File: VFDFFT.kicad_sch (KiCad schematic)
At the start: 278 parts, among them J1 USB_C_Receptacle_USB2.0, J10 Conn_01x02_Pin, J11 Conn_01x02_Male, J12 Conn_01x02_Male, J13 Conn_01x02_Male, J14 AudioJack3_Ground, J15 USB_C_Receptacle_USB2.0, J2 BATT, J3 FILAMENT+, J4 VFD_SIG, J5 USB_A, J6 Conn_01x03_Socket, J7 Conn_01x03_Socket, J8 Conn_01x02_Pin, J9 Conn_01x02_Pin, Q1 IRL7486MTRPBF, Q10 AO3400A, Q11 AO3400A, Q12 FS5N10S, Q2 ASDM30DN40E, Q3 ASDM30DN40E, Q4 HSCB2903, Q5 HSCB2903, Q6 AP6800, Q7 FS5N10S, Q8 FS5N10S, Q9 AO3400A, U1 IP2368, U10 TPS61170, U11 TPS61170, U12 W25Q128JVS, U13 TPS62170DSG, U14 LM358, U15 LM324, U16 LM3478, U17 LM2738, U18 ES9023, U19 CH340E, U2 78L05_SOT23, U3 TPS40305, U4 LM3478, U5 LM3478, U6 STM32F446VETx, U7 AP6181, U8 HDC1080, U9 OPT3001DNPR, X1 SX1M32.768KM10F30TNN, Y1 WTL3M45404LZ, Y2 24M

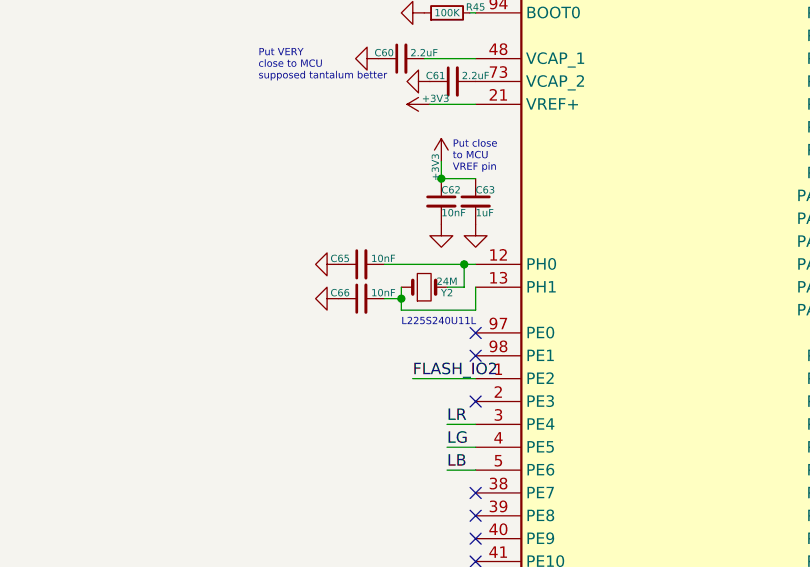
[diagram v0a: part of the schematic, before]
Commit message: file sync
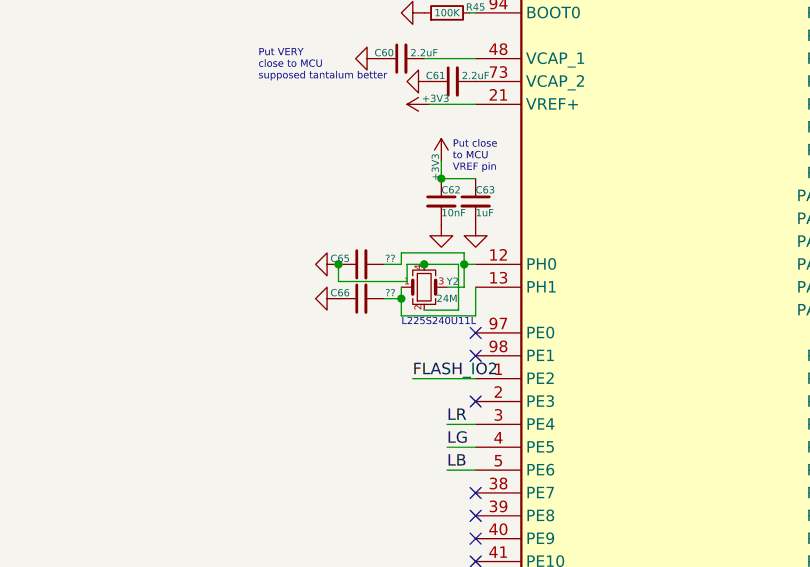
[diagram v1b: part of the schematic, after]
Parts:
- removed Y2: 24M, Resistor_SMD:R_0805_2012Metric, symbol Device:Crystal_Small
- added Y2: 24M, Crystal:Crystal_SMD_3225-4Pin_3.2x2.5mm, symbol Device:Crystal_GND24_Small
- C65, C66: value 10nF -> ??
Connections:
- net GND: now also Y2.2, Y2.4
- net at C66.2, U6.13 (PH1): now also Y2.1
- net at C65.2, U6.12 (PH0): now also Y2.3
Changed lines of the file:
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@@
   (junction (at 58.42 175.26) (diameter 0) (color 0 0 0 0)
   )
+  (junction (at 293.37 78.74) (diameter 0) (color 0 0 0 0)
+  )
   (junction (at 104.775 25.4) (diameter 0) (color 0 0 0 0)
   )
@@
   (junction (at 168.275 269.875) (diameter 0) (color 0 0 0 0)
   )
+  (junction (at 283.845 78.74) (diameter 0) (color 0 0 0 0)
+  )
   (junction (at 40.005 97.79) (diameter 0) (color 0 0 0 0)
   )
@@
     (stroke (width 0) (type default))
   )
+  (wire (pts (xy 291.465 78.74) (xy 291.465 80.645))
+    (stroke (width 0) (type default))
+  )
   (wire (pts (xy 199.39 241.935) (xy 202.565 241.935))
     (stroke (width 0) (type default))
@@
     (stroke (width 0) (type default))
   )
+  (wire (pts (xy 290.83 78.74) (xy 288.925 78.74))
+    (stroke (width 0) (type default))
+  )
   (wire (pts (xy 169.545 239.395) (xy 190.5 239.395))
     (stroke (width 0) (type default))
@@
     (stroke (width 0) (type default))
   )
-  (wire (pts (xy 299.085 81.28) (xy 299.085 83.82))
+  (wire (pts (xy 299.085 81.28) (xy 299.085 84.455))
     (stroke (width 0) (type default))
   )
@@
     (stroke (width 0) (type default))
   )
+  (wire (pts (xy 297.18 83.82) (xy 297.18 78.74))
+    (stroke (width 0) (type default))
+  )
   (wire (pts (xy 64.135 99.695) (xy 64.135 100.33))
     (stroke (width 0) (type default))
@@
     (stroke (width 0) (type default))
   )
+  (wire (pts (xy 293.37 78.74) (xy 291.465 78.74))
+    (stroke (width 0) (type default))
+  )
   (wire (pts (xy 75.565 119.38) (xy 75.565 121.92))
     (stroke (width 0) (type default))
@@
     (stroke (width 0) (type default))
   )
+  (wire (pts (xy 293.37 83.82) (xy 297.18 83.82))
+    (stroke (width 0) (type default))
+  )
   (wire (pts (xy 210.82 168.91) (xy 210.82 169.545))
     (stroke (width 0) (type default))
   )
+  (wire (pts (xy 297.815 77.47) (xy 297.815 78.74))
+    (stroke (width 0) (type default))
+  )
   (wire (pts (xy 175.26 275.59) (xy 187.96 275.59))
     (stroke (width 0) (type default))
@@
     (stroke (width 0) (type default))
   )
-  (wire (pts (xy 290.83 83.82) (xy 290.83 82.55))
+  (wire (pts (xy 290.83 84.455) (xy 290.83 82.55))
     (stroke (width 0) (type default))
   )
@@
     (stroke (width 0) (type default))
   )
+  (wire (pts (xy 283.845 80.645) (xy 283.845 78.74))
+    (stroke (width 0) (type default))
+  )
   (wire (pts (xy 57.15 111.76) (xy 57.15 112.395))
     (stroke (width 0) (type default))
@@
     (stroke (width 0) (type default))
   )
-  (wire (pts (xy 288.925 78.74) (xy 297.815 78.74))
+  (wire (pts (xy 290.83 77.47) (xy 297.815 77.47))
     (stroke (width 0) (type default))
   )
@@
     (stroke (width 0) (type default))
   )
+  (wire (pts (xy 290.83 77.47) (xy 290.83 78.74))
+    (stroke (width 0) (type default))
+  )
   (wire (pts (xy 295.275 116.84) (xy 299.085 116.84))
     (stroke (width 0) (type default))
@@
     (stroke (width 0) (type default))
   )
+  (wire (pts (xy 297.18 78.74) (xy 293.37 78.74))
+    (stroke (width 0) (type default))
+  )
   (wire (pts (xy 73.66 252.73) (xy 73.66 264.16))
     (stroke (width 0) (type default))
@@
     (stroke (width 0) (type default))
   )
-  (wire (pts (xy 299.085 83.82) (xy 290.83 83.82))
+  (wire (pts (xy 299.085 84.455) (xy 290.83 84.455))
     (stroke (width 0) (type default))
   )
@@
     (stroke (width 0) (type default))
   )
+  (wire (pts (xy 291.465 80.645) (xy 283.845 80.645))
+    (stroke (width 0) (type default))
+  )
   (wire (pts (xy 179.07 62.23) (xy 182.245 62.23))
     (stroke (width 0) (type default))
@@
     )
   )
-  (symbol (lib_id "Device:Crystal_Small") (at 293.37 81.28 0) (unit 1)
-    (in_bom yes) (on_board yes) (dnp no)
-    (property "Reference" "Y2" (at 295.91 81.915 0)
-      (effects (font (size 0.8 0.8)))
-    )
-    (property "Value" "24M" (at 295.91 80.645 0)
-      (effects (font (size 0.8 0.8)))
-    )
-    (property "Footprint" "Resistor_SMD:R_0805_2012Metric" (at 293.37 81.28 0)
-      (effects (font (size 1.27 1.27)) hide)
-    )
-    (property "Datasheet" "~" (at 293.37 81.28 0)
-      (effects (font (size 1.27 1.27)) hide)
-    )
-    (pin "1")
-    (pin "2")
-    (instances
-      (project "VFDFFT"
-        (path "/7a53a631-dec5-4274-9a20-e8f914b63ed5"
-          (reference "Y2") (unit 1)
-        )
-      )
-    )
-  )
   (symbol (lib_id "power:GND") (at 91.44 116.205 180) (unit 1)
     (in_bom yes) (on_board yes) (dnp no) (fields_autoplaced)
@@
       (effects (font (size 0.8 0.8)) (justify left))
     )
-    (property "Value" "10nF" (at 290.195 81.915 90)
+    (property "Value" "??" (at 290.195 81.915 90)
       (effects (font (size 0.8 0.8)) (justify left))
     )
@@
       (effects (font (size 0.8 0.8)) (justify left))
     )
-    (property "Value" "10nF" (at 290.195 78.105 90)
+    (property "Value" "??" (at 290.195 78.105 90)
       (effects (font (size 0.8 0.8)) (justify left))
     )
@@
         )
       )
+    )
+  )
+  (symbol (lib_id "Device:Crystal_GND24_Small") (at 293.37 81.28 0) (unit 1)
+    (in_bom yes) (on_board yes) (dnp no)
+    (property "Reference" "Y2" (at 296.545 80.645 0)
+      (effects (font (size 0.8 0.8)))
+    )
+    (property "Value" "24M" (at 295.91 82.55 0)
+      (effects (font (size 0.8 0.8)))
+    )
+    (property "Footprint" "Crystal:Crystal_SMD_3225-4Pin_3.2x2.5mm" (at 293.37 81.28 0)
+      (effects (font (size 1.27 1.27)) hide)
+    )
+    (property "Datasheet" "~" (at 293.37 81.28 0)
+      (effects (font (size 1.27 1.27)) hide)
+    )
+    (pin "1")
+    (pin "2")
+    (pin "3")
+    (pin "4")
+    (instances
+      (project "VFDFFT"
+        (path "/7a53a631-dec5-4274-9a20-e8f914b63ed5"
+          (reference "Y2") (unit 1)
+        )
+      )
